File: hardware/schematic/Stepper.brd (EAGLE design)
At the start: 100 x 80 mm, 34 parts, among them U16 MMSZ5225BT1G, U19 LM358DR

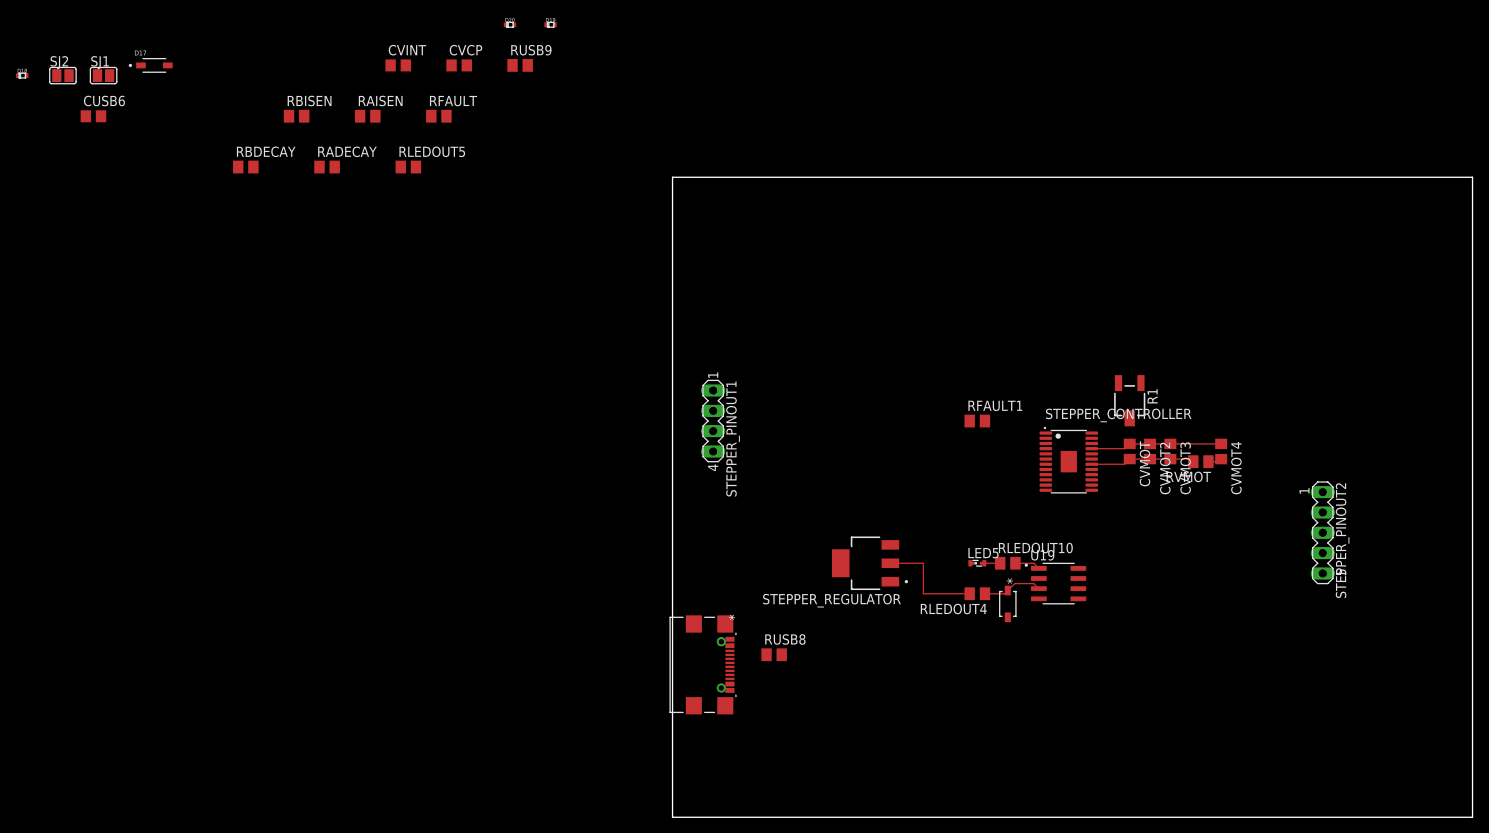
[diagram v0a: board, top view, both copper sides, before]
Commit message: Add files via upload
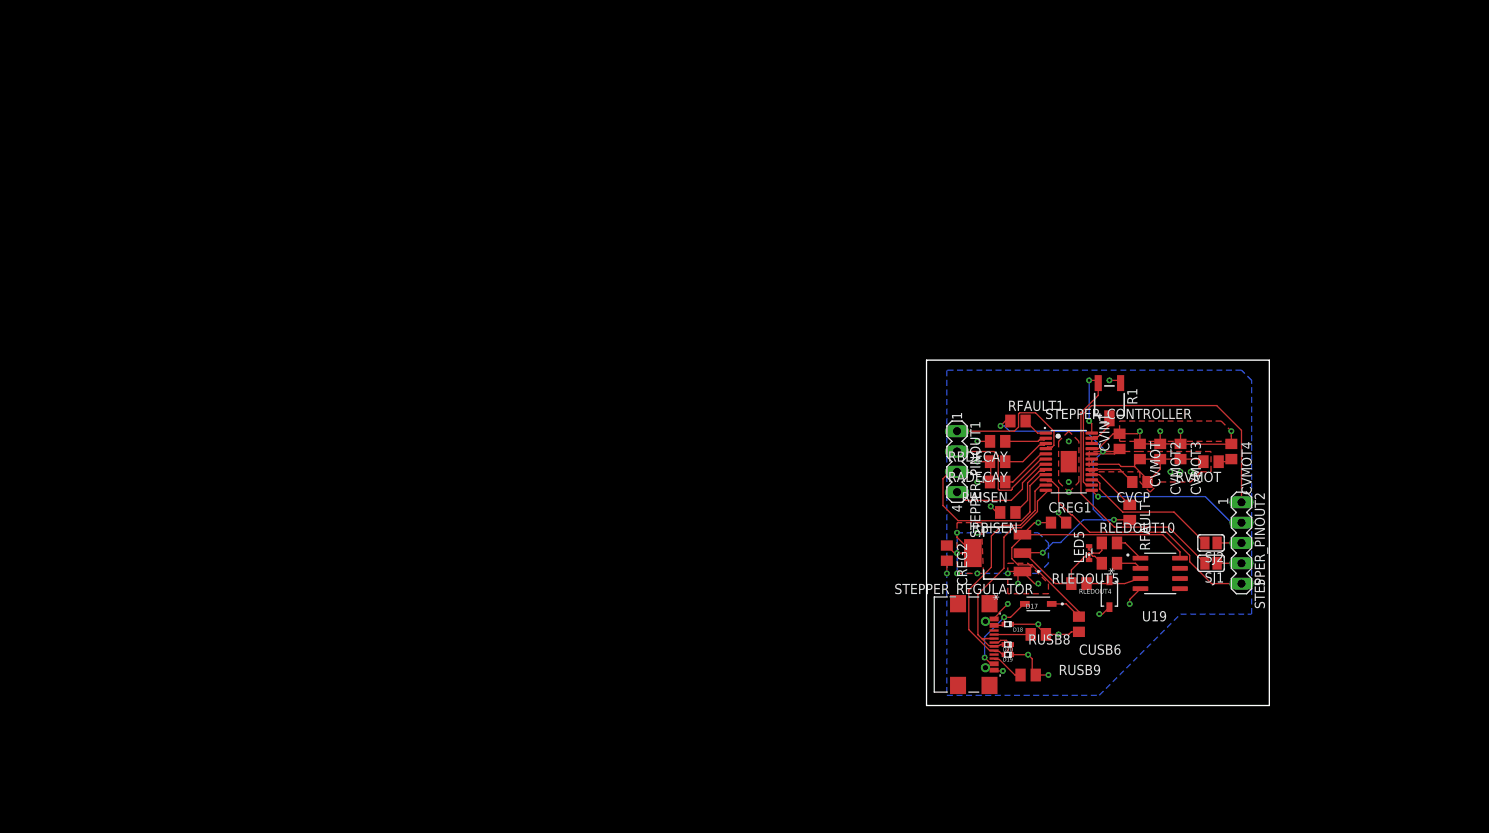
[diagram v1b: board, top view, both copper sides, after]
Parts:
- added CREG1: 10uF, rcl:C0805
- added CREG2: 22uF, rcl:C0805
- moved SJ2 154.9 mm to (67.3, 34.3), turned to 180 degrees
- moved SJ1 151.3 mm to (67.3, 31.8), turned to 180 degrees
- moved D18 141.0 mm to (41.9, 24.1), turned to 180 degrees
- moved CUSB6 138.6 mm to (50.8, 24.1), turned to 270 degrees
- moved D17 129.4 mm to (45.7, 26.7), turned to 180 degrees
- moved RBISEN 101.8 mm to (41.9, 38.1), turned to 180 degrees
- moved CVINT 101.7 mm to (55.9, 47.0), turned to 90 degrees
- moved RLEDOUT5 100.7 mm to (54.6, 31.8), turned to 180 degrees
- moved RBDECAY 100.0 mm to (40.6, 47.0), turned to 180 degrees
- moved CVCP 99.8 mm to (58.4, 41.9), turned to 180 degrees
- moved RFAULT 99.6 mm to (57.1, 38.1), turned to 270 degrees
- moved D20 99.4 mm to (41.9, 21.6), turned to 180 degrees
- moved RUSB9 99.2 mm to (44.5, 17.8)
- moved D19 97.3 mm to (41.9, 20.3), turned to 180 degrees
- moved RADECAY 91.6 mm to (40.6, 44.5), turned to 180 degrees
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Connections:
- removed net 5VOUTUSB22: CUSB6.1, CVCP.1, CVMOT.2, CVMOT2.2, CVMOT3.2, D17.C, RVMOT.2, STEPPER_CONTROLLER.18, STEPPER_CONTROLLER.19, STEPPER_REGULATOR.3, U19.8
- new net 5VOUTUSB2: CREG1.1, CUSB6.1, CVCP.1, CVMOT.2, CVMOT2.2, CVMOT3.2, D17.C, RVMOT.2, STEPPER_CONTROLLER.18, STEPPER_CONTROLLER.19, STEPPER_REGULATOR.3, U19.8
- net 3.3VOUTUSB2: now also CREG2.1, STEPPER_REGULATOR.4
- net GND: now also CREG1.2, CREG2.2
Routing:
- net 5VOUTUSB2: track 0.00 -> 66.3 mm, vias 0 -> 4
- net 3.3VOUTUSB2: track 13.7 -> 73.0 mm, vias 0 -> 9
- net GND: track 16.4 -> 69.5 mm, vias 0 -> 25
- net VREF: track 0.00 -> 41.8 mm, vias 0 -> 2
- net N$37: track 0.00 -> 40.2 mm
- net GPIO8M: track 0.00 -> 33.2 mm
- net N$90: track 0.00 -> 31.4 mm
- net GPIO9M: track 0.00 -> 29.6 mm
- net N$30: track 0.00 -> 23.4 mm
- net N$38: track 0.00 -> 20.4 mm, vias 0 -> 1
- net N$28: track 0.00 -> 17.9 mm
- net N$36: track 0.00 -> 17.9 mm
- net N$29: track 0.00 -> 17.3 mm
- net N$31: track 0.00 -> 13.9 mm
- net 5VOUTUSB22: track 13.1 -> 0.00 mm
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- added copper zone on layer 1, net 3.3VOUTUSB2
- added copper zone on layer 16, net 3.3VOUTUSB2
- added copper zone on layer 1, net 5VOUTUSB2
- added copper zone on layer 1, net GND
- added copper zone on layer 16, net GND
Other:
- board size 100 x 80 mm -> 42.8 x 43.2 mm
